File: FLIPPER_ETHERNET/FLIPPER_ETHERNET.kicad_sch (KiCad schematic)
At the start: 26 parts, among them J1 RJ45_Hanrun_HR911105A_Horizon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, J2 Conn_01x08_Socket, J3 Conn_01x10_Socket, SW1 SW_Push, U1 ENC28J60x-ML, Y1 25MHz

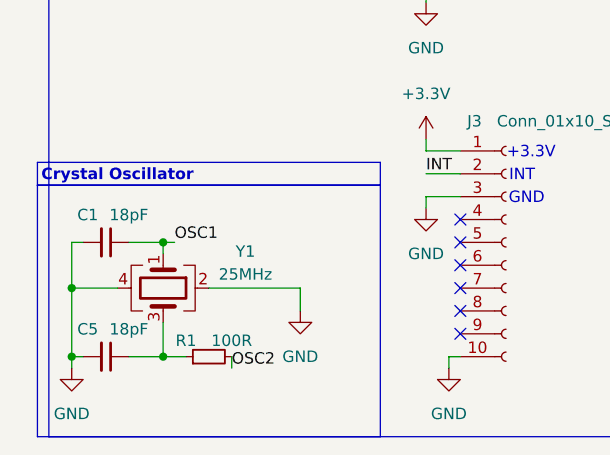
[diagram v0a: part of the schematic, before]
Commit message: feat: some pcb routes corrected
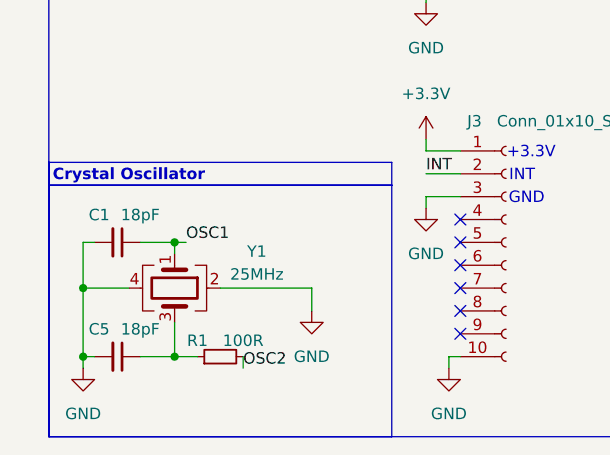
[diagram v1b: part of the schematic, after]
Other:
- moved on the sheet: C1, C5, R1, Y1
